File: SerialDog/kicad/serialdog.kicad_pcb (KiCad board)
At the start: 2 copper layers, 72.4 x 39.4 mm, 24 parts, among them J1 Connector:USB_C_Receptacle, J2 1x6_2.54_smd_header, U1 USBLC6-2SC6, U2 Interface_USB:CP2102N-A01-GQF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

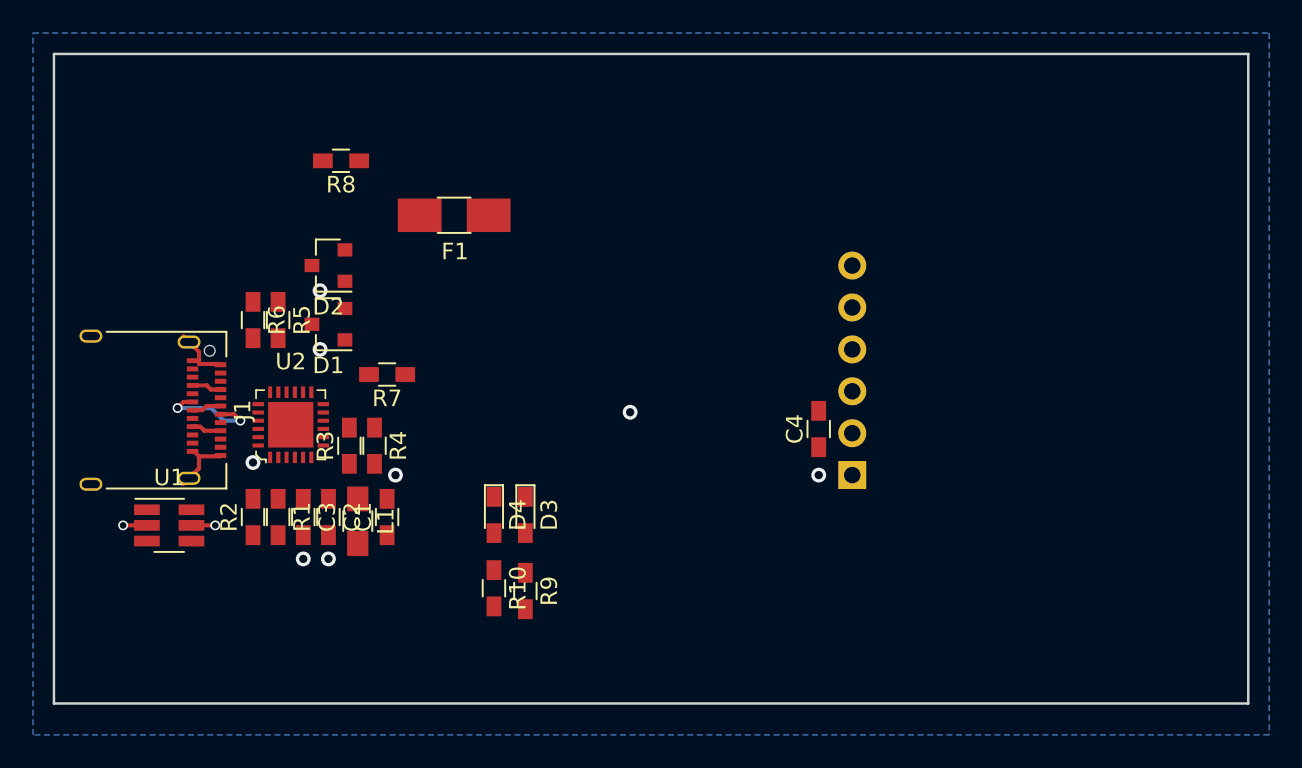
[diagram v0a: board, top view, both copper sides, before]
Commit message: Made first pcb layout draft
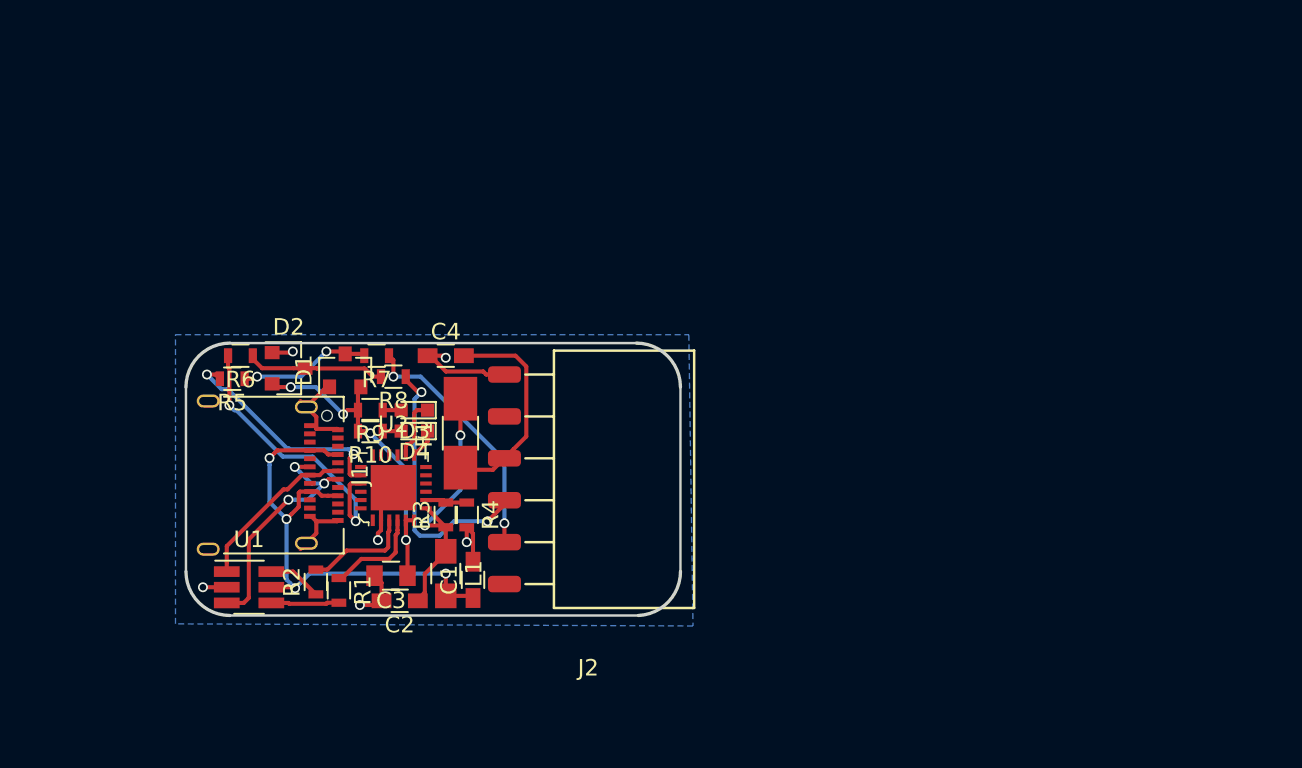
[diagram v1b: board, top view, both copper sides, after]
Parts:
- C3: footprint Resistors_SMD:R_0603_HandSoldering -> Capacitors_SMD:C_0805
- D3, D4: footprint LEDs:LED_0603_HandSoldering -> LEDs:LED_0603
- J2: footprint Pin_Headers:Pin_Header_Angled_1x06_Pitch2.54mm -> uart-adapters:1x6 header female smd; moved to F.Cu
- R1, R10, R2, R3, R4, R5, R6, R7, R8, R9: footprint Resistors_SMD:R_0603_HandSoldering -> Resistors_SMD:R_0603
- moved C4 23.0 mm to (133.6, 85.0), turned to 0 degrees
- moved J2 21.1 mm to (137.2, 92.5)
- moved R9 14.4 mm to (129.0, 88.3), turned to 180 degrees
- moved R8 13.5 mm to (130.4, 86.2)
- moved F1 13.2 mm to (134.5, 89.7), turned to 90 degrees
- moved R10 12.1 mm to (129.0, 89.5), turned to 180 degrees
- moved D3 9.25 mm to (131.7, 88.3), turned to 180 degrees
- moved J1 8.13 mm to (122.0, 92.2)
- moved U2 7.30 mm to (130.4, 93.0)
- moved R3 7.19 mm to (133.6, 94.6)
- moved D4 7.01 mm to (131.7, 89.5), turned to 180 degrees
- moved R4 6.98 mm to (134.9, 94.6)
- moved D2 6.67 mm to (124.1, 85.7), turned to 0 degrees
- moved C2 6.67 mm to (130.8, 99.8), turned to 180 degrees
- moved C1 6.45 mm to (135.3, 98.6)
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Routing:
- net /VBUS: track 5.05 -> 31.4 mm, vias 1 -> 4
- net Net-(C3-Pad1): track 0.00 -> 20.9 mm, vias 0 -> 4
- net GND: track 8.79 -> 28.1 mm, vias 9 -> 6
- net Net-(R6-Pad2): track 0.00 -> 17.4 mm, vias 0 -> 2
- net /REGIN: track 0.00 -> 16.7 mm, vias 0 -> 2
- net Net-(J2-Pad4): track 0.00 -> 16.6 mm, vias 0 -> 2
- net Net-(J2-Pad5): track 0.00 -> 15.3 mm, vias 0 -> 2
- net Net-(R5-Pad2): track 0.00 -> 14.0 mm, vias 0 -> 2
- net /VOUT: track 0.00 -> 13.1 mm
- net Net-(J1-PadA7): track 6.55 -> 15.0 mm, vias 2 -> 3
- net /TX: track 0.00 -> 8.41 mm
- net Net-(J1-PadA6): track 1.84 -> 10.2 mm
- net /RX: track 0.00 -> 7.73 mm, vias 0 -> 2
- net Net-(R2-Pad2): track 0.00 -> 6.61 mm
- net Net-(R1-Pad1): track 0.00 -> 6.08 mm
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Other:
- board size 72.4 x 39.4 mm -> 30 x 16.5 mm
